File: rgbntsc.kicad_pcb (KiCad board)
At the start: 2 copper layers, 50 x 70 mm, 53 parts, among them J1 USB_C_Receptacle_Power, J2 VGA, J3 SCART_CONN, J4 Mini-DIN-4, U1 LM1881, U2 74AHCT1G86, U3 74AHCT1G86, U4 SC6206B-65K5, U5 CXA2075, U6 TPF144-VR, X1 O32253579545MHEA4SI

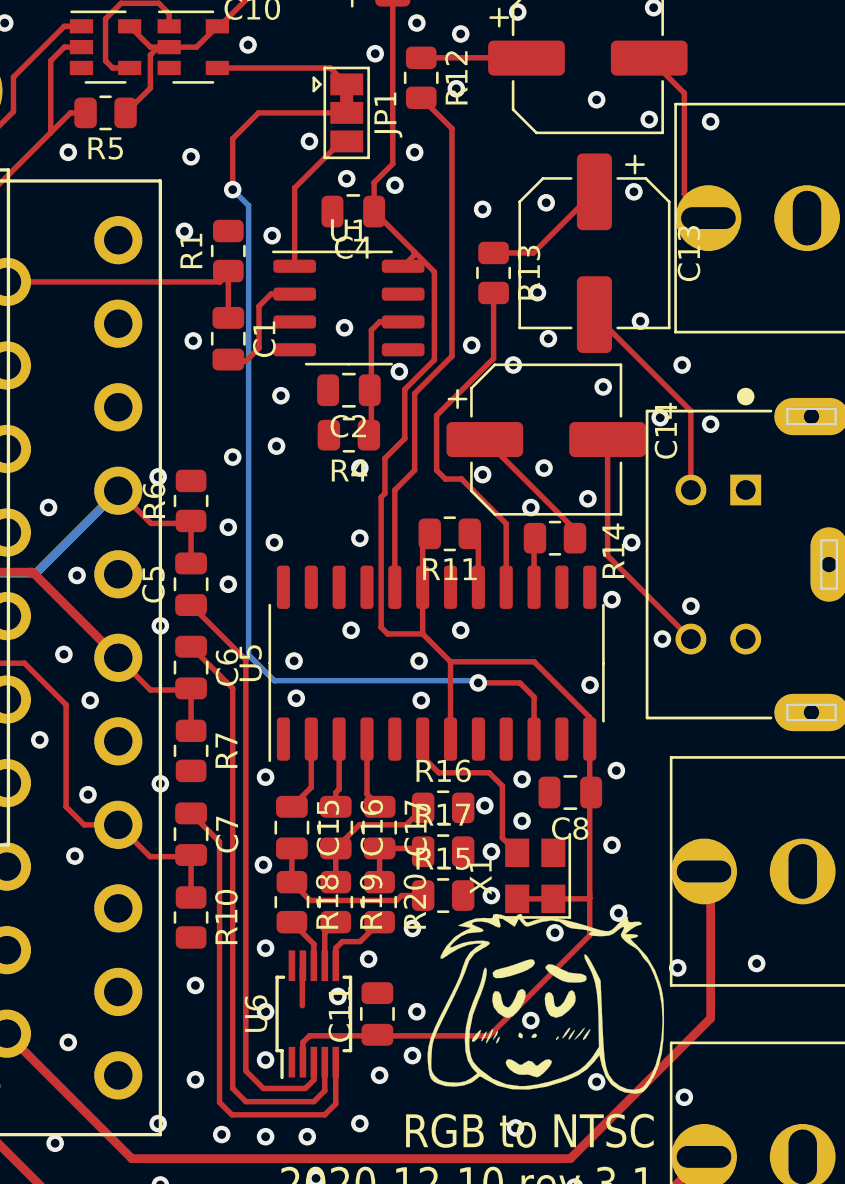
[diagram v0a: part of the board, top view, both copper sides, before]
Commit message: corrected components
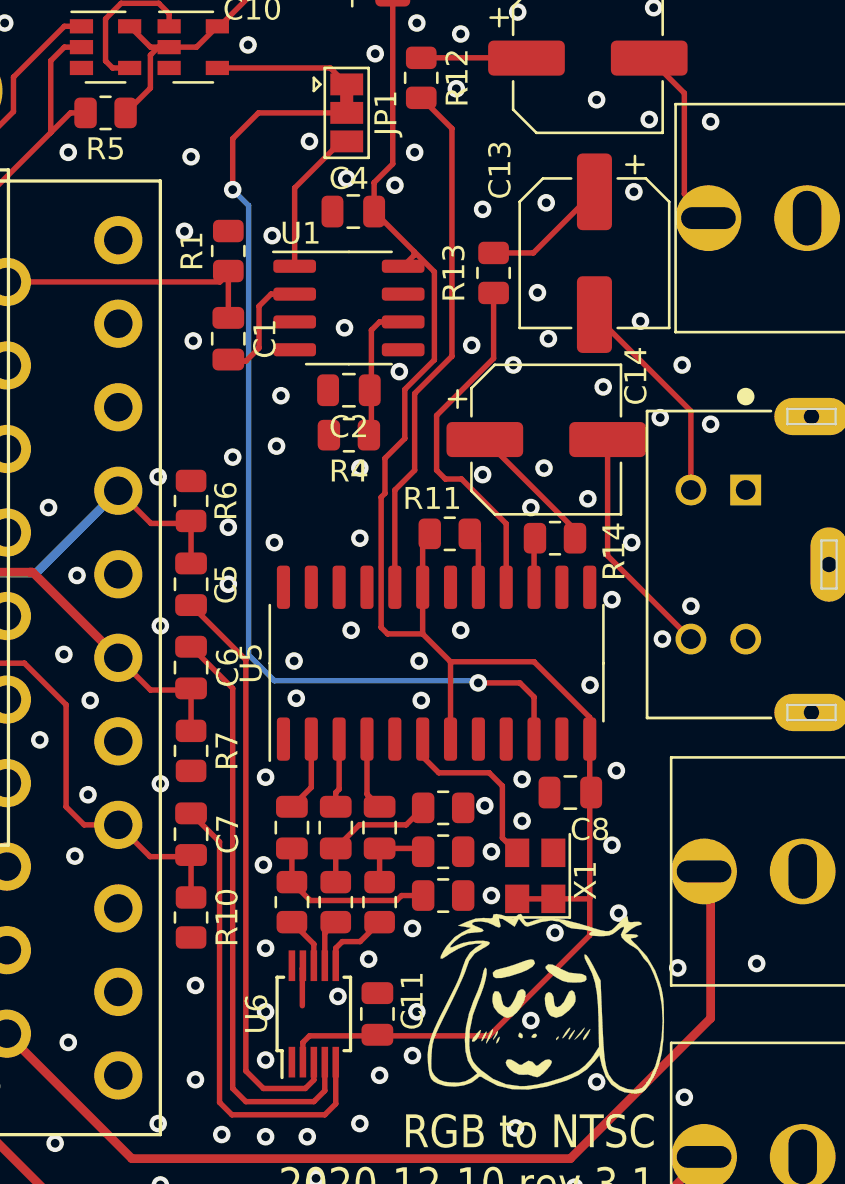
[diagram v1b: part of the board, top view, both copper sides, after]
